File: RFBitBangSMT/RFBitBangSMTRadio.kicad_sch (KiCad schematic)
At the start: 138 parts, among them J10 si5351mod, J12 Conn_Coaxial, J17 Filt1, J18 Filt2, Q1 MMBT3904, Q10 MMBT3904, Q11 MMBT3904, Q12 MMBT3904, Q13 SS8550, Q15 NC, Q2 MMBT3904, Q3 2N7000, Q5 NC, Q6 2N7000, Q7 2N7000, Q8 SS8550, Q9 2N7000, T1 Trifilar, T2 Trifilar, T3 Current, U4 LM358, U6 SI5351A, Y2 7.X MHz, Y3 25 MHz, Y4 7.X MHz, Y5 7.X MHz

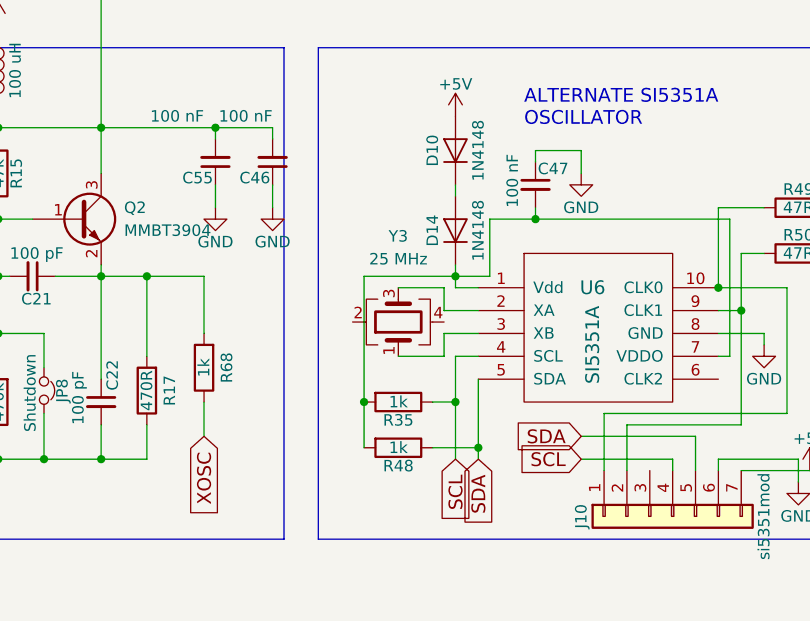
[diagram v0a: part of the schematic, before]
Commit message: Added TCXO option to RFBitBanger SMT
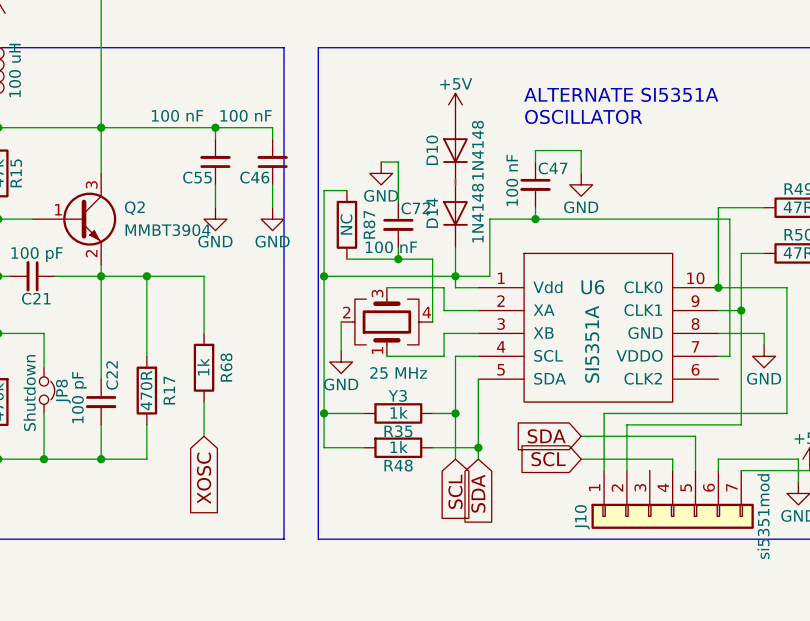
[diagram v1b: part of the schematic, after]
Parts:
- added C72: 100 nF, Capacitor_SMD:C_0805_2012Metric_Pad1.18x1.45mm_HandSolder, symbol RFBitBangSMT-rescue:C_Small
- added R87: NC, Resistor_THT:R_Axial_DIN0207_L6.3mm_D2.5mm_P7.62mm_Horizontal, symbol RFBitBangSMT-rescue:R
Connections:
- net GND: now also Y3.2, C72.1
- net at C47.2, D14.1 (K), R35.2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: now also R87.2
- net at Y3.4: now also C72.2, R87.1
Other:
- moved on the sheet: D14, R35, Y3
